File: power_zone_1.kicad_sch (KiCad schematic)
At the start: 1 part, among them U2 TPS74801DRC

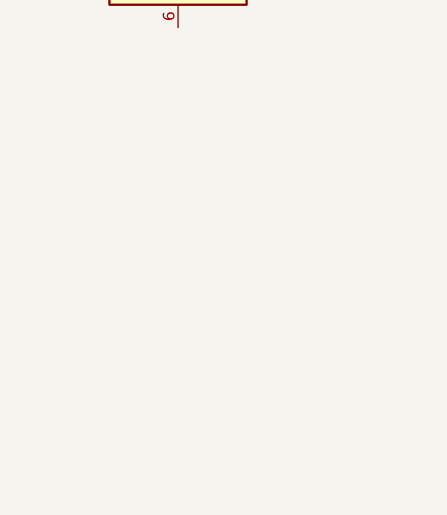
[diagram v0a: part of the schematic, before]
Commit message: progress
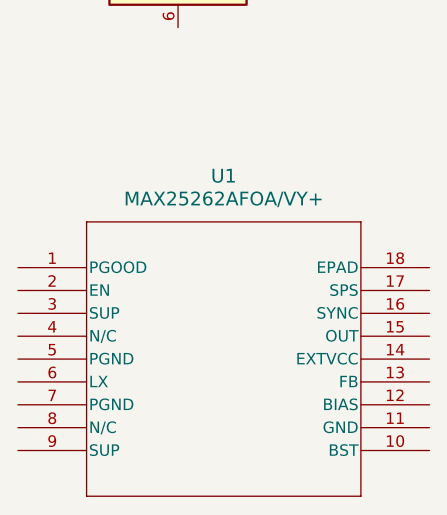
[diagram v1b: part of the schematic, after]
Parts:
- added U1: MAX25262AFOA/VY+, MAX25262:21-100429_90-100162_MXM, symbol MAX25262:MAX25262AFOA_VY+
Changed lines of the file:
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@@
+				)
+			)
+			(project "power_zone_1"
+				(path "/9810aa7e-84d2-47e9-b179-0eeb14854ddb"
+					(reference "U2")
+					(unit 1)
 				)
 			)
 		)
 	)
+	(symbol
+		(lib_id "MAX25262:MAX25262AFOA_VY+")
+		(at 24.13 76.2 0)
+		(unit 1)
+		(exclude_from_sim no)
+		(in_bom yes)
+		(on_board yes)
+		(dnp no)
+		(fields_autoplaced yes)
+		(property "Reference" "U1"
+			(at 46.99 66.04 0)
+			(effects
+				(font
+					(size 1.524 1.524)
+				)
+			)
+		)
+		(property "Value" "MAX25262AFOA/VY+"
+			(at 46.99 68.58 0)
+			(effects
+				(font
+					(size 1.524 1.524)
+				)
+			)
+		)
+		(property "Footprint" "MAX25262:21-100429_90-100162_MXM"
+			(at 24.13 76.2 0)
+			(effects
+				(font
+					(size 1.27 1.27)
+					(italic yes)
+				)
+				(hide yes)
+			)
+		)
+		(property "Datasheet" "MAX25262AFOA/VY+"
+			(at 24.13 76.2 0)
+			(effects
+				(font
+					(size 1.27 1.27)
+					(italic yes)
+				)
+				(hide yes)
+			)
+		)
+		(property "Description" ""
+			(at 24.13 76.2 0)
+			(effects
+				(font
+					(size 1.27 1.27)
+				)
+				(hide yes)
+			)
+		)
+		(pin "16"
+		)
+		(pin "3"
+		)
+		(pin "4"
+		)
+		(pin "9"
+		)
+		(pin "12"
+		)
+		(pin "14"
+		)
+		(pin "1"
+		)
+		(pin "2"
+		)
+		(pin "7"
+		)
+		(pin "6"
+		)
+		(pin "11"
+		)
+		(pin "10"
+		)
+		(pin "18"
+		)
+		(pin "13"
+		)
+		(pin "15"
+		)
+		(pin "5"
+		)
+		(pin "8"
+		)
+		(pin "17"
+		)
+		(instances
+			(project ""
+				(path "/6f2a77a4-5c51-4809-903e-53c484a031d8/08ce249e-3973-46ed-9801-faf01e378b6f"
+					(reference "U3")
+					(unit 1)
+				)
+			)
+			(project "power_zone_1"
+				(path "/9810aa7e-84d2-47e9-b179-0eeb14854ddb"
+					(reference "U1")
+					(unit 1)
+				)
+			)
+		)
+	)
+	(sheet_instances
+		(path "/"
+			(page "1")
+		)
+	)
+	(embedded_fonts no)
 )

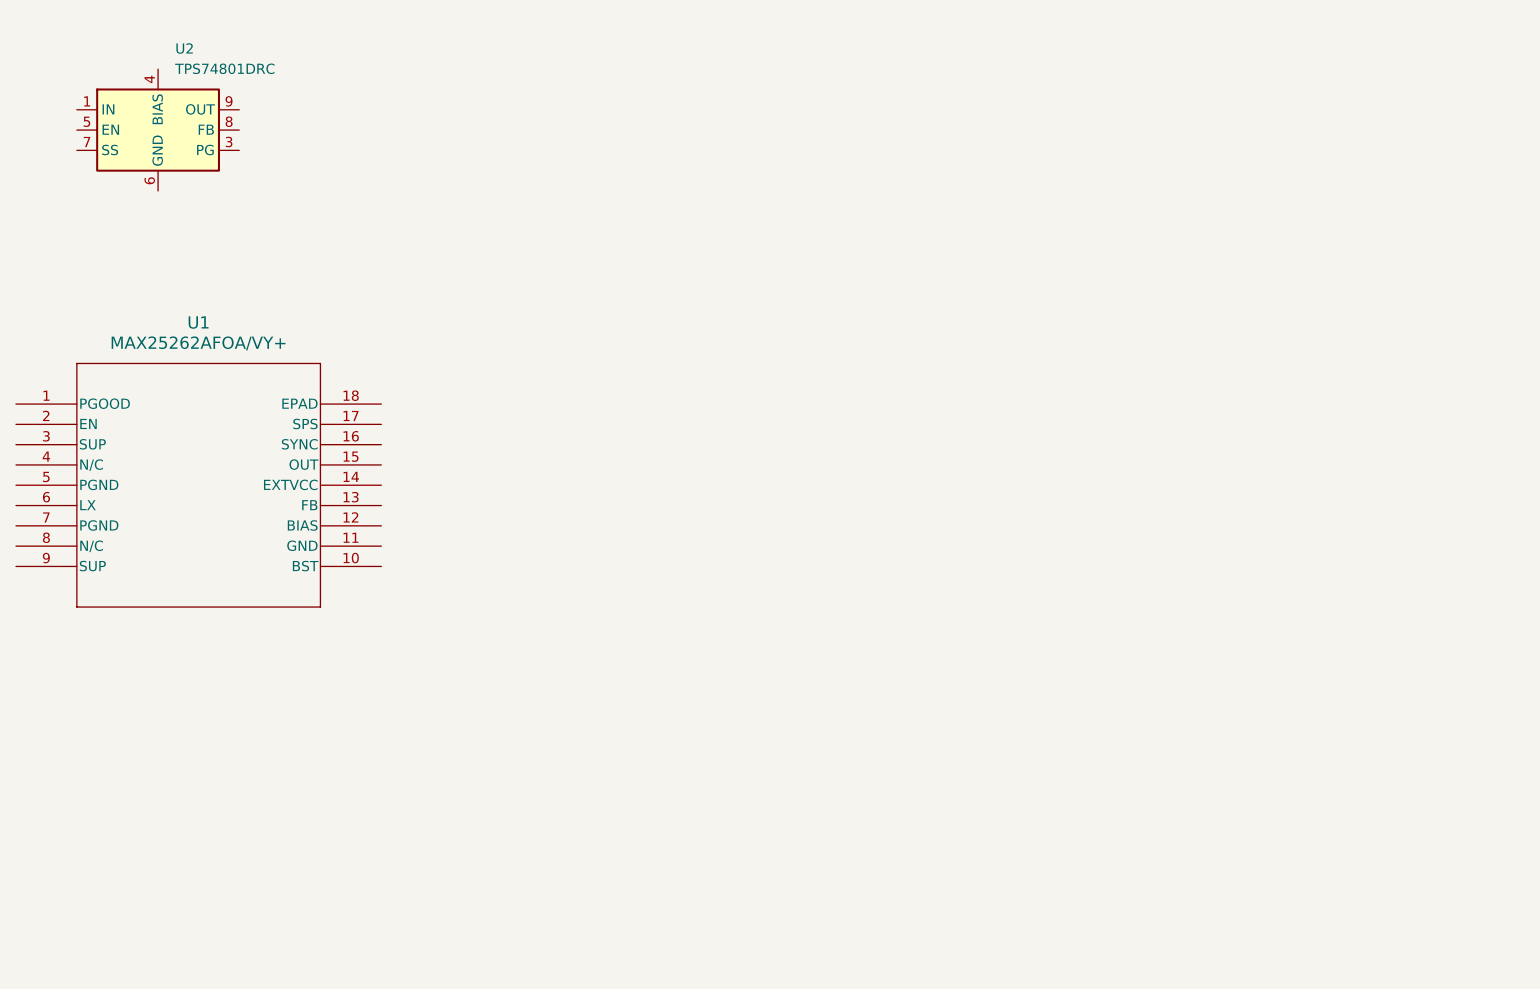
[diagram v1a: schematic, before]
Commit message: power zone 1 updates
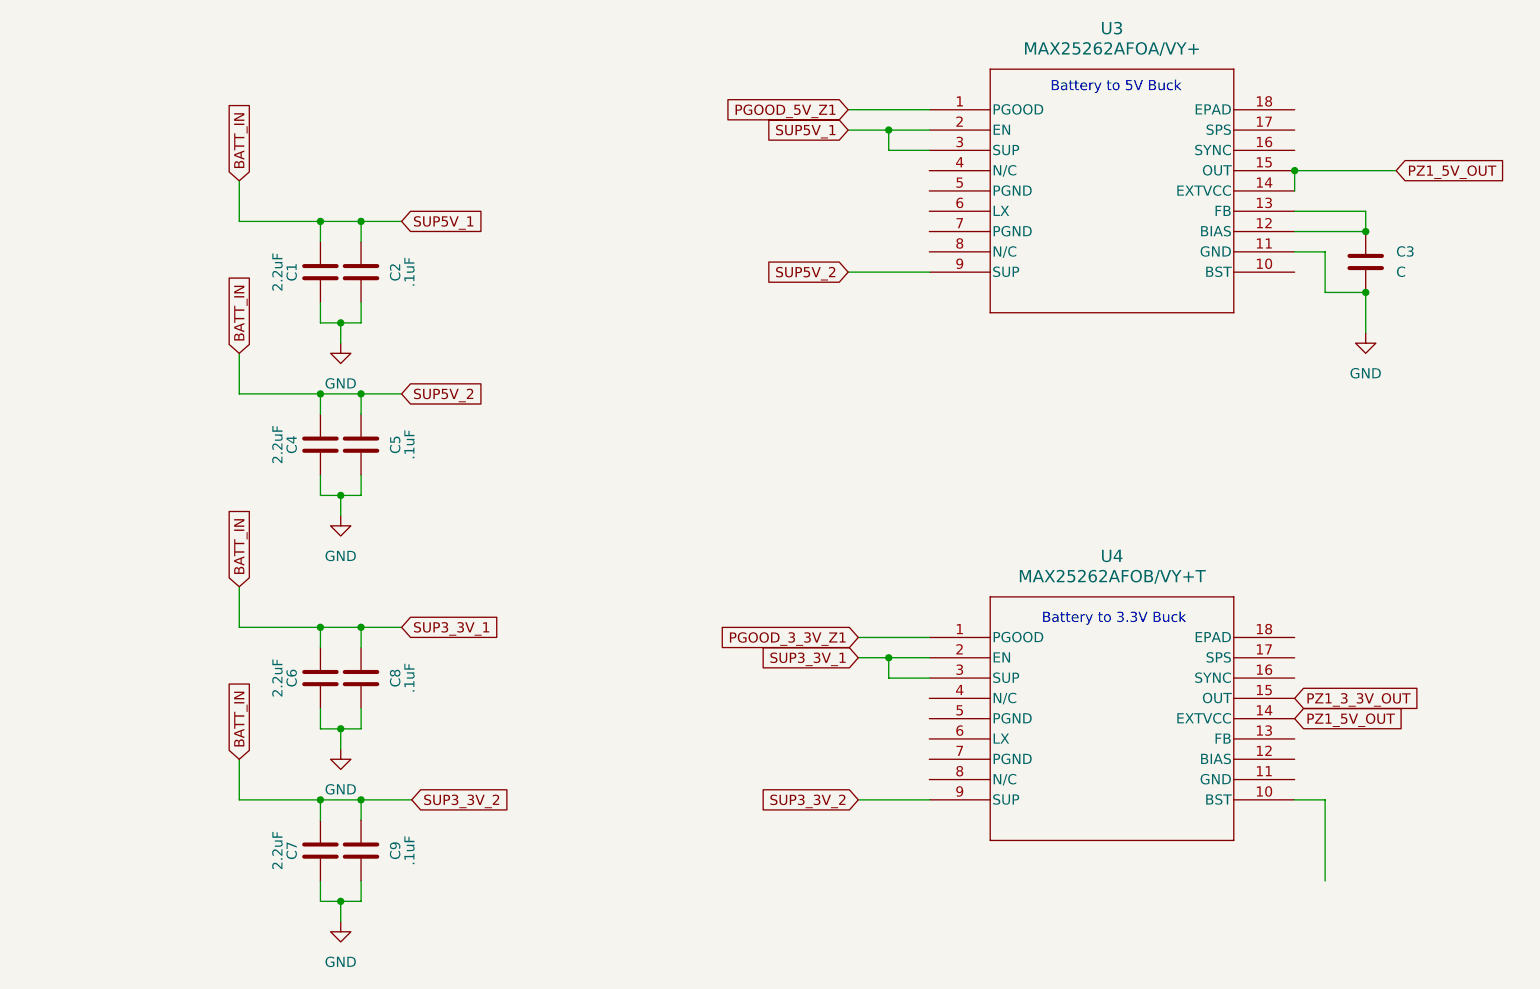
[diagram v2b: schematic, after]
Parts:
- removed U2: TPS74801DRC, Package_SON:VSON-10-1EP_3x3mm_P0.5mm_EP1.65x2.4mm_ThermalVias, symbol Regulator_Linear:TPS74801DRC
- added C1, C4, C6, C7: 2.2uF, Capacitor_SMD:C_0805_2012Metric, symbol Device:C
- added C2, C5, C8, C9: .1uF, Capacitor_SMD:C_0805_2012Metric, symbol Device:C
- added C3: C, symbol Device:C
- added U4: MAX25262AFOB/VY+T, 21-100429_90-100162_MXM, symbol MAX25262AFOB:MAX25262AFOB_VY+T
- renumbered U1 to U3
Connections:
- net PGOOD_5V_Z1: now reaches U3.1 (PGOOD)
- net GND: now reaches U3.11 (GND)
- net GND: now also C1.1, C2.1, C3.2, C4.1, C5.1, C6.1, C7.1, C8.1, C9.1
- net at U3.12 (BIAS): now also U3.13 (FB), C3.1
- net PZ1_5V_OUT: now reaches U3.14 (EXTVCC)
- net PZ1_5V_OUT: now also U3.15 (OUT), U4.14 (EXTVCC)
- net BATT_IN: now reaches U3.2 (EN)
- net BATT_IN: now also U3.3 (SUP), U3.9 (SUP), C1.2, C2.2, C4.2, C5.2, C6.2, C7.2, C8.2, C9.2, U4.2 (EN), U4.3 (SUP), U4.9 (SUP)
- new net PGOOD_3_3V_Z1: U4.1 (PGOOD)
- new net PZ1_3_3V_OUT: U4.15 (OUT)
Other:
- note added: "Battery to 3.3V Buck"
- note added: "Battery to 5V Buck"
- moved on the sheet: U3

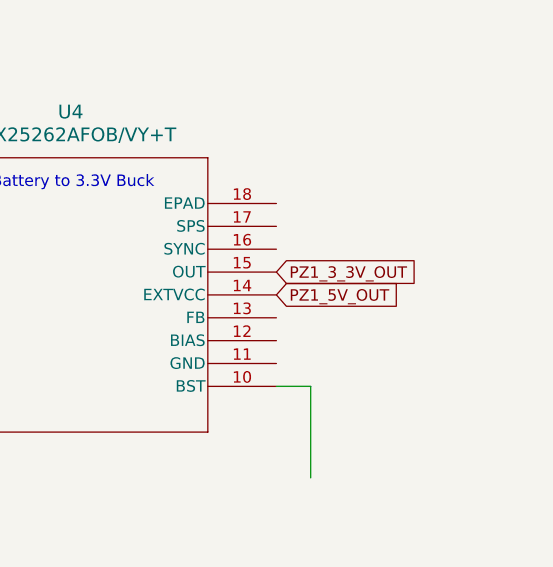
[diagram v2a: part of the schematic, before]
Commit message: progress
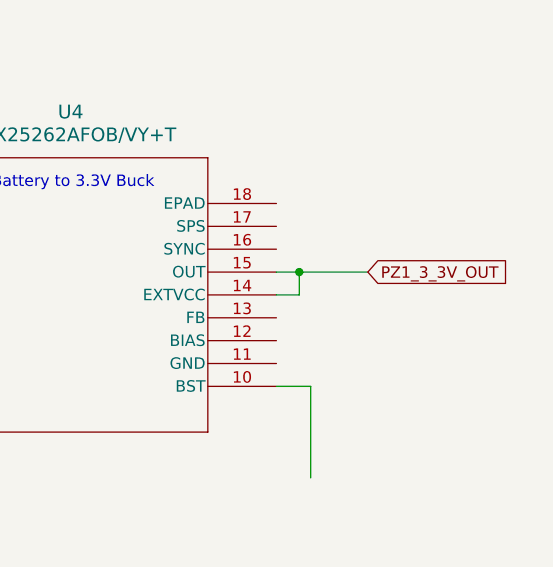
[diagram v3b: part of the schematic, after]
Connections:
- net PZ1_3_3V_OUT: now also U4.14 (EXTVCC)
- net PZ1_5V_OUT: no longer U4.14 (EXTVCC)
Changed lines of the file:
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@@
+	)
+	(junction
+		(at 186.69 113.03)
+		(diameter 0)
+		(color 0 0 0 0)
 	)
 	(junction
@@
 	(wire
 		(pts
+			(xy 194.31 113.03) (xy 186.69 113.03)
+		)
+		(stroke
+			(width 0)
+			(type default)
+		)
+	)
+	(wire
+		(pts
+			(xy 186.69 113.03) (xy 184.15 113.03)
+		)
+		(stroke
+			(width 0)
+			(type default)
+		)
+	)
+	(wire
+		(pts
 			(xy 128.27 41.91) (xy 133.35 41.91)
 		)
@@
 	(wire
 		(pts
+			(xy 184.15 115.57) (xy 186.69 115.57)
+		)
+		(stroke
+			(width 0)
+			(type default)
+		)
+	)
+	(wire
+		(pts
 			(xy 62.23 55.88) (xy 62.23 53.34)
 		)
@@
 	(wire
 		(pts
+			(xy 186.69 115.57) (xy 186.69 113.03)
+		)
+		(stroke
+			(width 0)
+			(type default)
+		)
+	)
+	(wire
+		(pts
 			(xy 64.77 66.04) (xy 64.77 68.58)
 		)
@@
 	(global_label "PZ1_3_3V_OUT"
 		(shape input)
-		(at 184.15 113.03 0)
+		(at 194.31 113.03 0)
 		(fields_autoplaced yes)
 		(effects
@@
 		)
 		(property "Intersheetrefs" "${INTERSHEET_REFS}"
-			(at 200.8632 113.03 0)
+			(at 211.0232 113.03 0)
 			(effects
 				(font
@@
 			(effects
 				(font
-					(size 1.27 1.27)
-				)
-				(justify left)
-				(hide yes)
-			)
-		)
-	)
-	(global_label "PZ1_5V_OUT"
-		(shape input)
-		(at 184.15 115.57 0)
-		(fields_autoplaced yes)
-		(effects
-			(font
-				(size 1.27 1.27)
-			)
-			(justify left)
-		)
-		(property "Intersheetrefs" "${INTERSHEET_REFS}"
-			(at 198.6861 115.57 0)
-			(effects
-				(font
